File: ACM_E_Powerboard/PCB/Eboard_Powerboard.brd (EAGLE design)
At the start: 41.9 x 53 mm, 21 parts, among them IC1 TCMD4000, Q1 NGD8201ANT4G, Q2 NGD8201ANT4G, Q3 NGD8201ANT4G

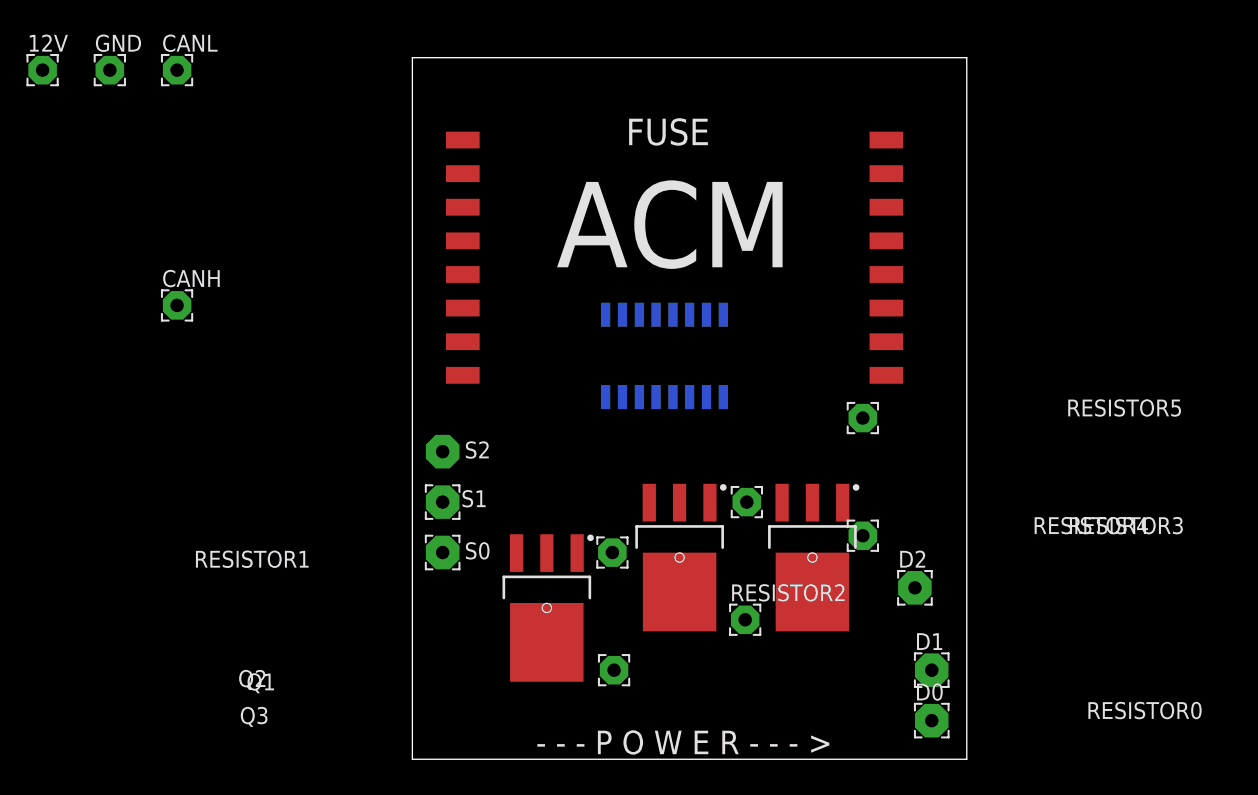
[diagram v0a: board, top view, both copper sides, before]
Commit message: Powerboard RDY
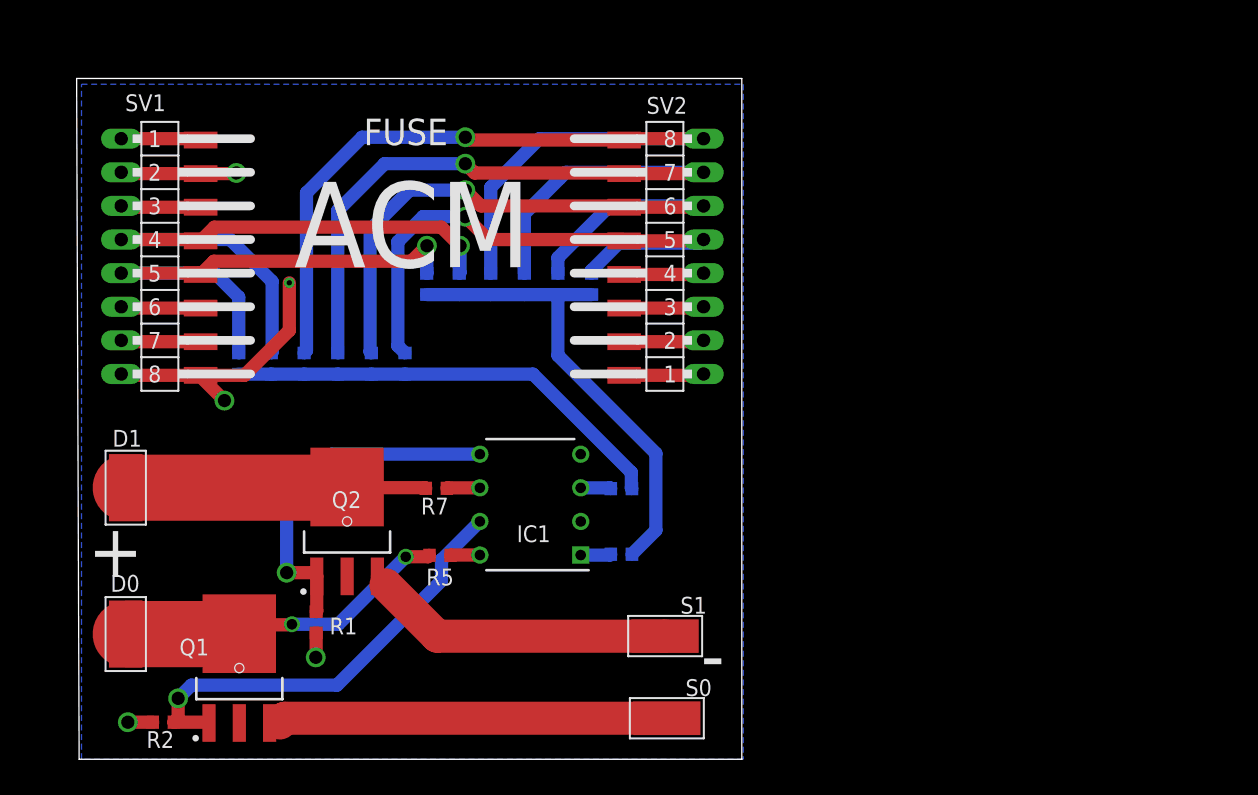
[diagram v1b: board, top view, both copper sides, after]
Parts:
- removed 12V, CANH, CANL, GND, RESISTOR0, RESISTOR1, RESISTOR2, RESISTOR3, RESISTOR4, RESISTOR5: (no value), wirepad:2,15/1,0
- removed D2, S2: (no value), wirepad:2,54/1,0
- removed Q3: NGD8201ANT4G, NGD8201ANT4G_Mosfet:TO229P990X238-4N
- added M0_AD0, M0_AD1, M0_AD2, M0_AD3, M0_PWM0, M0_PWM1, M1_AD0, M1_AD1, M1_AD2, M1_AD3, M1_PWM0, M1_PWM1, R1, R2: (no value), ERA-3AEB2262V(0603 Resistor):RESC1608X55N
- added R3, R4: 200 Ohm, ERA-3AEB2262V(0603 Resistor):RESC1608X55N
- added R5, R7: 1K Ohm, ERA-3AEB2262V(0603 Resistor):RESC1608X55N
- added SV1, SV2: (no value), con-lstb:MA08-1W
- D0, D1, S0, S1: device wirepad:2,54/1,0 -> wirepad:5-2,5
- IC1: value TCMD4000 -> Optocoupler DIP; device SFH6916:SOIC127P695X210-16N -> TLP350(F):DIP762W60P254L966H485Q8N
- Q1, Q2: value NGD8201ANT4G -> (none)
- moved D1 62.4 mm to (-21.7, 20.5), turned to 180 degrees
- moved D0 61.3 mm to (-21.7, 9.46)
- moved Q2 25.3 mm to (-4.93, 18.0), turned to 90 degrees
- moved Q1 23.7 mm to (-13.1, 6.89), turned to 90 degrees
- moved S0 21.1 mm to (19.2, 3.10), turned to 90 degrees
- moved U$1 19.8 mm to (-16.0, 25.4)
- moved S1 19.6 mm to (19.1, 9.31), turned to 90 degrees
- moved IC1 15.1 mm to (8.91, 19.2), flipped to the top, turned to 180 degrees
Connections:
- removed net D0: D0.1, Q1.4
- removed net DRAIN2: D2.1, Q3.4
- removed net GATE2: Q3.1, RESISTOR5.1, U$1.I/O_AD0
- removed net SOURCE2: Q3.3, S2.1
- new net AD0: M0_AD0.2, M1_AD0.2, SV2.8, U$1.I/O_AD0
- new net AD1: M0_AD1.2, M1_AD1.2, SV2.7, U$1.I/O_AD1
- new net AD2: M0_AD2.2, M1_AD2.2, SV2.6, U$1.I/O_AD2_SDA
- new net AD3: M0_AD3.2, M1_AD3.2, SV2.5, U$1.I/O_AD3_SCL
- new net DRAIN0: D0.1, Q1.4, R5.2
- new net N$1: SV1.3, U$1.5V
- new net N$10: SV2.3, U$1.MOSI
- new net N$11: SV2.2, U$1.SCK
- new net N$12: SV2.1, U$1.5V1
- new net N$13: IC1.6, R7.1
- new net N$15: M0_AD0.1, M0_AD1.1, M0_AD2.1, M0_AD3.1, M0_PWM0.1, M0_PWM1.1, R3.2
- new net N$16: M1_AD0.1, M1_AD1.1, M1_AD2.1, M1_AD3.1, M1_PWM0.1, M1_PWM1.1, R4.2
- new net N$2: IC1.1, R3.1
- new net N$6: IC1.3, R4.1
- new net N$7: IC1.8, R5.1
- new net N$9: SV2.4, U$1.MISO
- new net PWM0: M0_PWM0.2, M1_PWM0.2, SV1.4, U$1.PWM0
- new net PWM1: M0_PWM1.2, M1_PWM1.2, SV1.5, U$1.PWM1_INT1
- net DRAIN1: now also R7.2
- net GATE0: now also IC1.7, R2.1; no longer RESISTOR1.1, U$1.PWM0
- net GATE1: now also IC1.5, R1.1; no longer RESISTOR3.1, U$1.PWM1_INT1
- net GND: now also IC1.2, IC1.4, R1.2, R2.2, SV1.2, SV1.8; no longer GND.1, RESISTOR0.1, RESISTOR2.1, RESISTOR4.1
- net N$3: now also SV1.1; no longer 12V.1
- net N$4: now also SV1.6; no longer CANL.1
- net N$5: now also SV1.7; no longer CANH.1
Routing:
- net AD0: track 0.00 -> 68.1 mm, vias 0 -> 1
- net AD1: track 0.00 -> 59.6 mm, vias 0 -> 1
- net AD2: track 0.00 -> 50.2 mm, vias 0 -> 1
- net PWM0: track 0.00 -> 46.9 mm, vias 0 -> 1
- net AD3: track 0.00 -> 43.0 mm, vias 0 -> 1
- net PWM1: track 0.00 -> 40.0 mm, vias 0 -> 1
- net N$15: track 0.00 -> 35.9 mm
- net N$16: track 0.00 -> 34.0 mm
- net GATE0: track 0.00 -> 33.9 mm, vias 0 -> 1
- net GND: track 0.00 -> 32.9 mm, vias 0 -> 5
- net SOURCE0: track 0.00 -> 30.8 mm
- net GATE1: track 0.00 -> 26.6 mm, vias 0 -> 1
- net DRAIN0: track 0.00 -> 25.4 mm, vias 0 -> 2
- net SOURCE1: track 0.00 -> 23.6 mm
- net DRAIN1: track 0.00 -> 22.8 mm
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- added copper zone on layer 16, net GND
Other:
- board size 41.9 x 53 mm -> 50.3 x 51.4 mm
- board text added: "+"
- board text added: "-"
- board text removed: "- - - P O W E R - - - >"
